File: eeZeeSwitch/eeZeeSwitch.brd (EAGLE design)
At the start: 15.7 x 7.6 mm, 6 parts

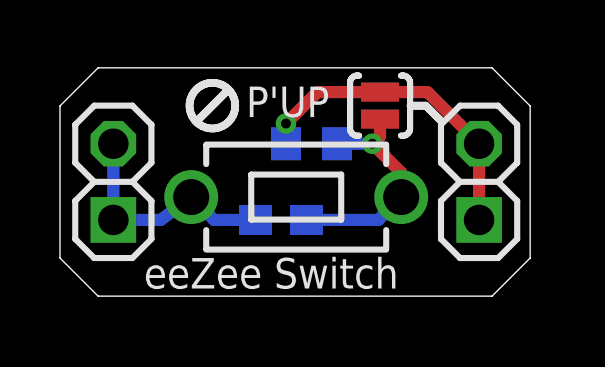
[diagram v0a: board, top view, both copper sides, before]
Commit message: Rev 0.1
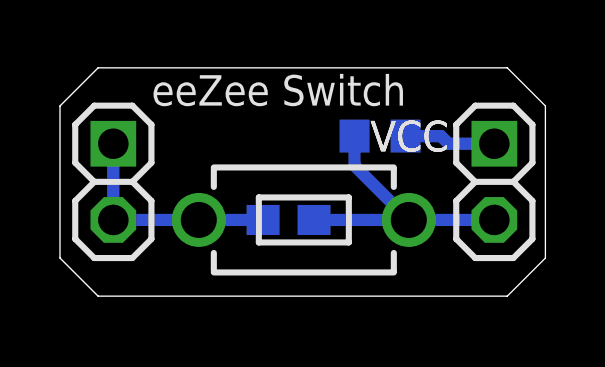
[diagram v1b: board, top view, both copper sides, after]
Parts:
- removed SJ1: P'UP, SparkFun:SJ_2S-NO
- moved R1 2.30 mm to (10.7, 5.33), turned to 180 degrees
- moved S1 0.80 mm to (8.13, 2.54)
- moved JP1 0.51 mm to (14.5, 3.81), turned to 270 degrees
- moved C1 0.25 mm to (7.62, 2.54)
- turned JP2 to 270 degrees
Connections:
- net N$1: now also JP1.2; no longer SJ1.1
- net N$3: no longer JP1.2, SJ1.2
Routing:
- net N$3: track 10.8 -> 3.07 mm, vias 1 -> 0
- net N$1: track 7.76 -> 9.55 mm, vias 1 -> 0
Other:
- board size 15.7 x 7.6 mm -> 16.2 x 7.6 mm
- board text added: "VCC"
- board text removed: "P'UP"
